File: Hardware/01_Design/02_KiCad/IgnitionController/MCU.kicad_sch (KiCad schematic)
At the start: 40 parts, among them U12 STM32F407VGTx, Y2 32.768kHz, Y3 8MHz

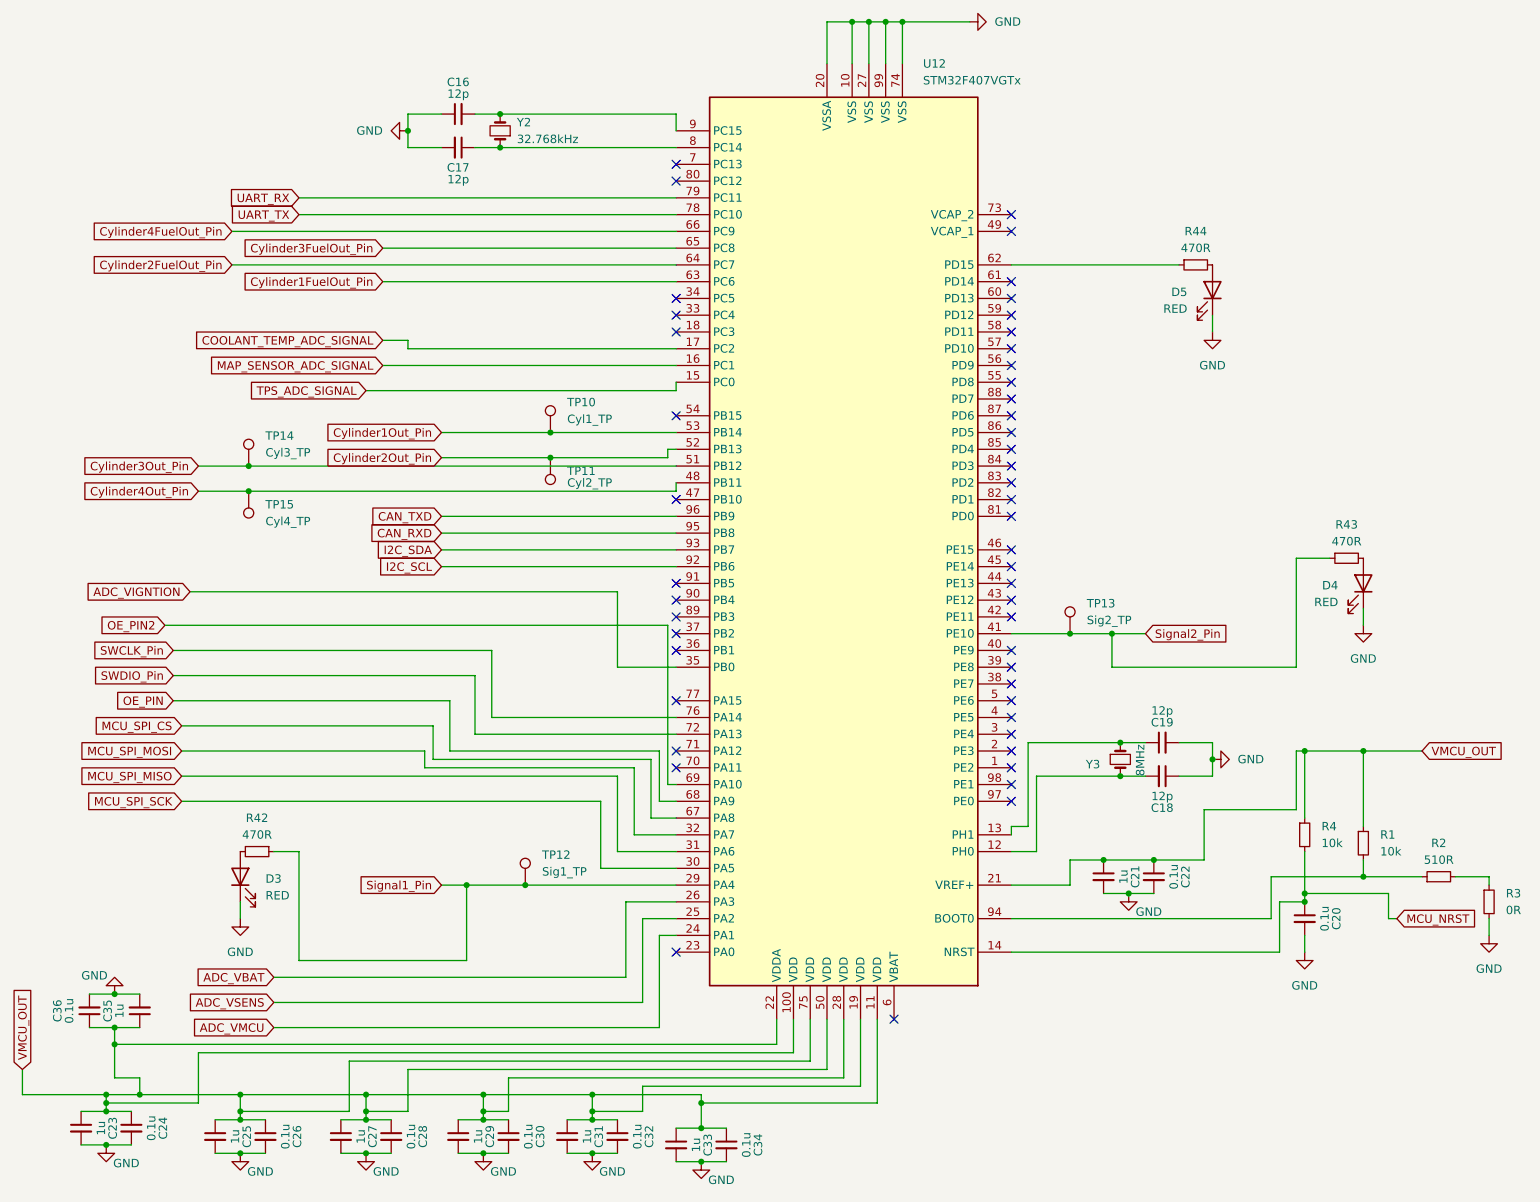
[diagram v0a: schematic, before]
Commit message: MCU HW Initial Layout
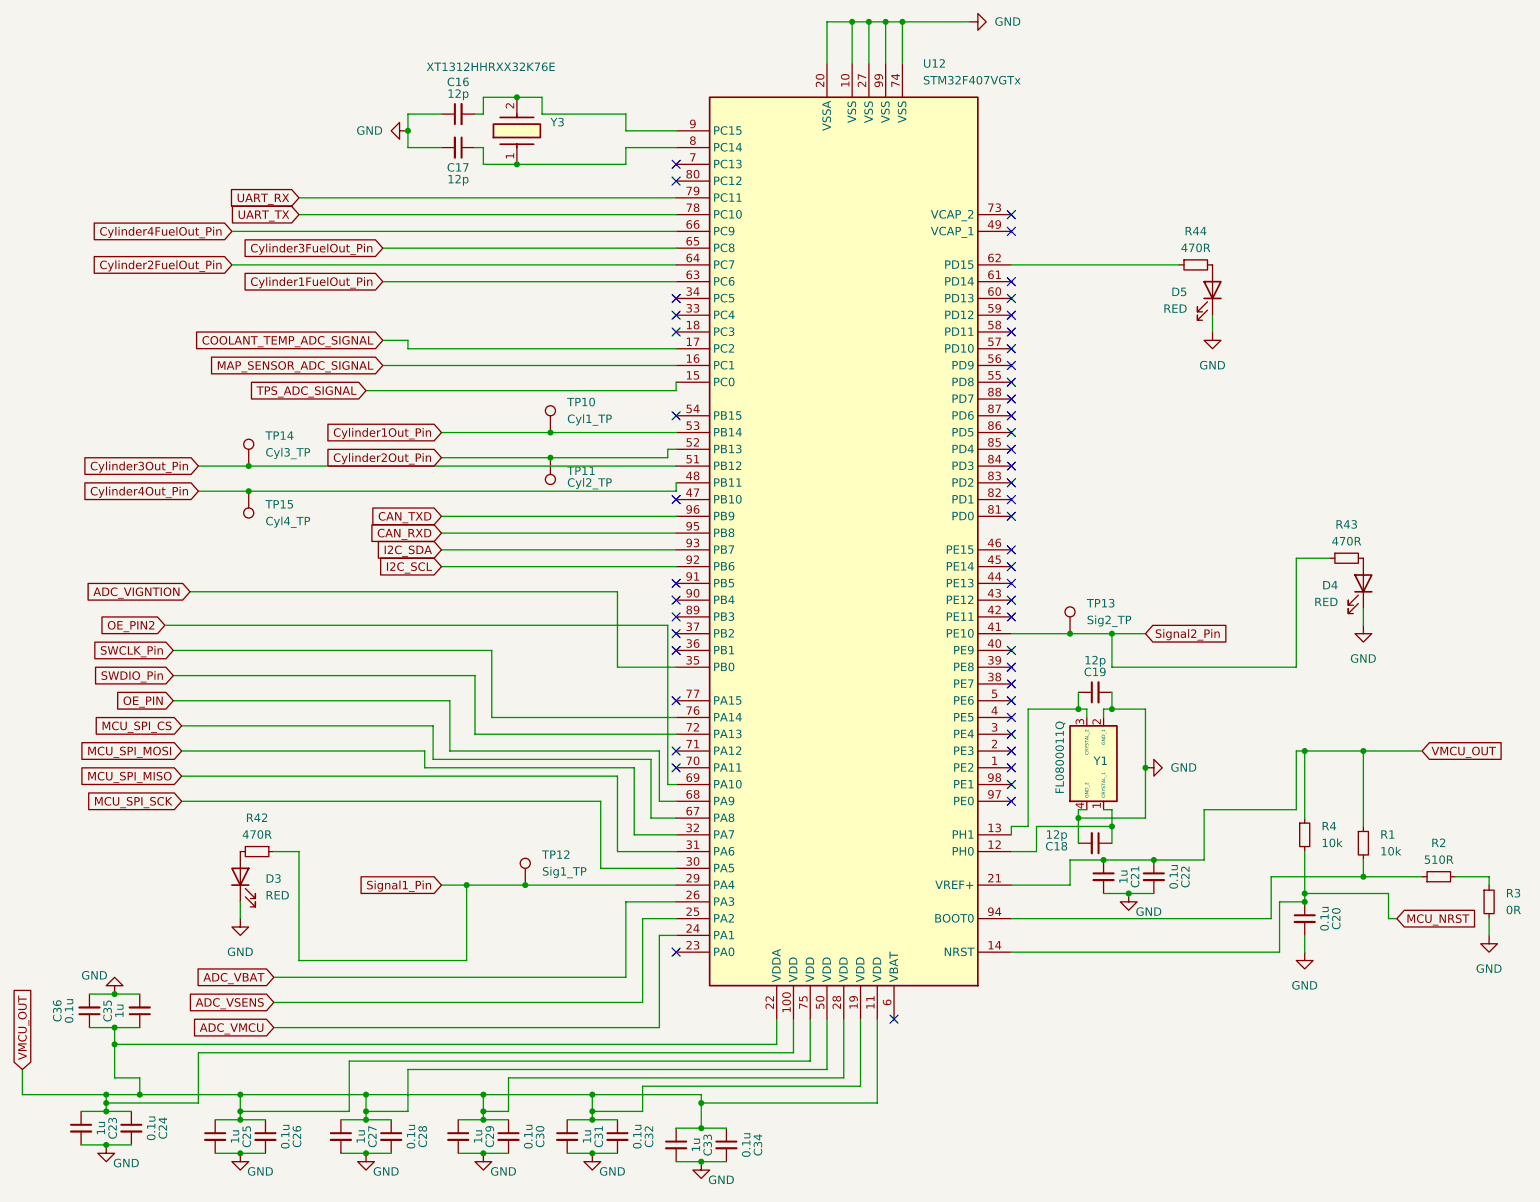
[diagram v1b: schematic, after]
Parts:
- removed Y2: 32.768kHz, Crystal:Crystal_HC52-8mm_Horizontal, symbol Device:Crystal_Small
- removed Y3: 8MHz, Crystal:Crystal_HC52-8mm_Horizontal, symbol Device:Crystal_Small
- added Y1: FL0800011Q, FL0800011Q, symbol FL0800011Q:FL0800011Q
- added Y3: XT1312HHRXX32K76E, XT1312HHRXX32K76E, symbol XT1312HHRXX32K76E:XT1312HHRXX32K76E
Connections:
- net GND: now also C18.2, Y1.2 (GND_1), Y1.4 (GND_2); no longer C18.1
- net at U12.12 (PH0): now also C18.1, Y1.1 (CRYSTAL_1); no longer C18.2
- net at C17.1, U12.8 (PC14): now also Y3.1
- net at C16.2, U12.9 (PC15): now also Y3.2
- net at C19.1, U12.13 (PH1): now also Y1.3 (CRYSTAL_2)
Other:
- moved on the sheet: C18, C19
